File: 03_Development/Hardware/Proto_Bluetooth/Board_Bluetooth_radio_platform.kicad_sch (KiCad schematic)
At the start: 51 parts, among them J1 Conn_01x02, J10 Conn_01x03, J11 HMI_rotaryEncoder_1, J12 HMI_rotaryEncoder_1, J13 Conn_01x08_epaper, J17 Conn_01x02, J19 Conn_01x02_rn52_usb, J2 Conn_01x08, J3 BT_RN52_connector_left, J4 Conn_01x02, J5 BT_RN52_connector_right, J6 FM_interface, J7 BT_debug_connector, J8 BT_extension_connector, J9 SYS_debug_connector, SW1 SW_Push, U1 LM317_TO-220, U2 NXE2S1205MC

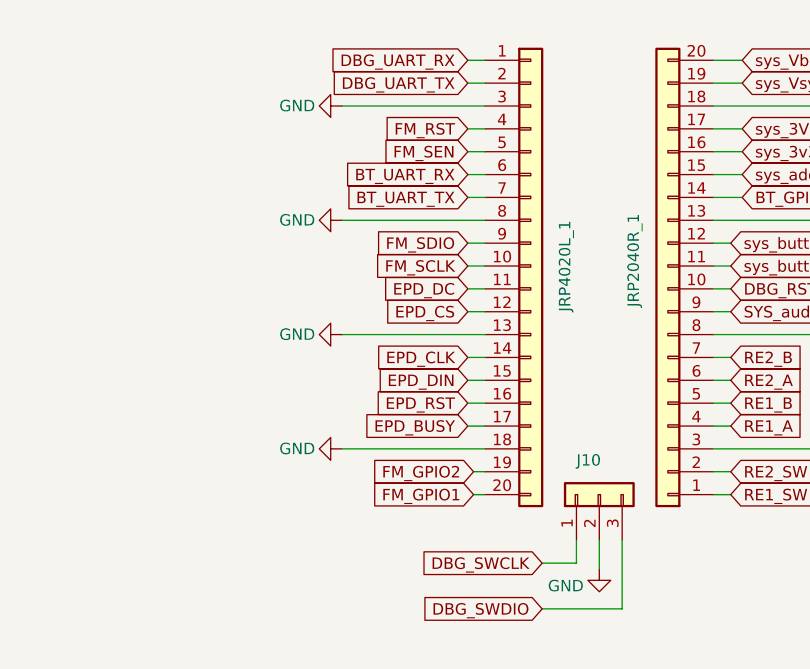
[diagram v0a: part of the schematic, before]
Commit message: [HDW_41] FIX communication lines to central unit
FM, EP and BT modules had been routed to ports of RP2040 which don't allow
UART or I2C and must have been changed
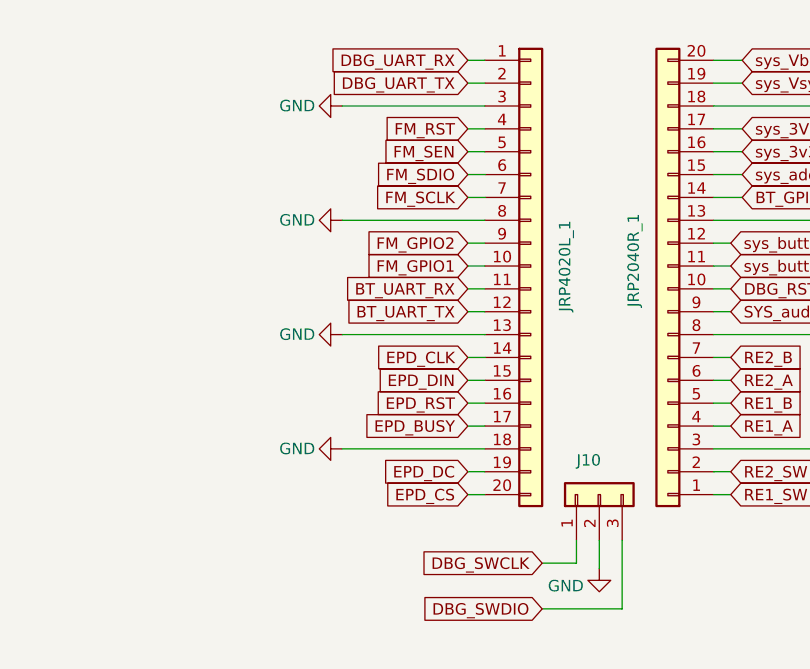
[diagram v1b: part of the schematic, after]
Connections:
- net BT_UART_RX: now also JRP4020L_1.11 (Pin_11); no longer JRP4020L_1.6 (Pin_6)
- net BT_UART_TX: now also JRP4020L_1.12 (Pin_12); no longer JRP4020L_1.7 (Pin_7)
- net EPD_CS: now also JRP4020L_1.20 (Pin_20); no longer JRP4020L_1.12 (Pin_12)
- net EPD_DC: now also JRP4020L_1.19 (Pin_19); no longer JRP4020L_1.11 (Pin_11)
- net FM_GPIO1: now also JRP4020L_1.10 (Pin_10); no longer JRP4020L_1.20 (Pin_20)
- net FM_GPIO2: now also JRP4020L_1.9 (Pin_9); no longer JRP4020L_1.19 (Pin_19)
- net FM_SCLK: now also JRP4020L_1.7 (Pin_7); no longer JRP4020L_1.10 (Pin_10)
- net FM_SDIO: now also JRP4020L_1.6 (Pin_6); no longer JRP4020L_1.9 (Pin_9)
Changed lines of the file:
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@@
     (stroke (width 0) (type default) (color 0 0 0 0))
   )
-  (wire (pts (xy 224.155 146.05) (xy 225.425 146.05))
+  (wire (pts (xy 223.52 146.05) (xy 225.425 146.05))
     (stroke (width 0) (type default) (color 0 0 0 0))
   )
@@
     (stroke (width 0) (type default) (color 0 0 0 0))
   )
-  (wire (pts (xy 224.155 148.59) (xy 225.425 148.59))
+  (wire (pts (xy 223.52 148.59) (xy 225.425 148.59))
     (stroke (width 0) (type default) (color 0 0 0 0))
   )
@@
     (stroke (width 0) (type default) (color 0 0 0 0))
   )
+  (global_label "BT_UART_RX" (shape input) (at 223.52 125.73 180) (fields_autoplaced)
+    (effects (font (size 1.27 1.27)) (justify right))
+    (property "Intersheet References" "${INTERSHEET_REFS}" (id 0) (at 209.7979 125.6506 0)
+      (effects (font (size 1.27 1.27)) (justify right) hide)
+    )
+  )
   (global_label "BT_SPI_SS" (shape input) (at 59.69 178.435 0) (fields_autoplaced)
     (effects (font (size 1.27 1.27)) (justify left))
@@
     )
   )
-  (global_label "BT_UART_RX" (shape input) (at 223.52 113.03 180) (fields_autoplaced)
-    (effects (font (size 1.27 1.27)) (justify right))
-    (property "Intersheet References" "${INTERSHEET_REFS}" (id 0) (at 209.7979 112.9506 0)
-      (effects (font (size 1.27 1.27)) (justify right) hide)
-    )
-  )
   (global_label "FM_SDIO" (shape input) (at 91.44 182.88 180) (fields_autoplaced)
     (effects (font (size 1.27 1.27)) (justify right))
@@
     )
   )
+  (global_label "FM_GPIO1" (shape input) (at 223.52 123.19 180) (fields_autoplaced)
+    (effects (font (size 1.27 1.27)) (justify right))
+    (property "Intersheet References" "${INTERSHEET_REFS}" (id 0) (at 211.9145 123.1106 0)
+      (effects (font (size 1.27 1.27)) (justify right) hide)
+    )
+  )
   (global_label "sys_3V3_EN" (shape input) (at 254 107.95 0) (fields_autoplaced)
     (effects (font (size 1.27 1.27)) (justify left))
@@
     )
   )
-  (global_label "EPD_DC" (shape input) (at 223.52 125.73 180) (fields_autoplaced)
-    (effects (font (size 1.27 1.27)) (justify right))
-    (property "Intersheet References" "${INTERSHEET_REFS}" (id 0) (at 213.9102 125.6506 0)
-      (effects (font (size 1.27 1.27)) (justify right) hide)
-    )
-  )
   (global_label "BT_SPKR_R+" (shape input) (at 59.944 145.415 0) (fields_autoplaced)
     (effects (font (size 1.27 1.27)) (justify left))
@@
     )
   )
-  (global_label "EPD_CS" (shape input) (at 223.52 128.27 180) (fields_autoplaced)
-    (effects (font (size 1.27 1.27)) (justify right))
-    (property "Intersheet References" "${INTERSHEET_REFS}" (id 0) (at 213.9707 128.1906 0)
-      (effects (font (size 1.27 1.27)) (justify right) hide)
-    )
-  )
   (global_label "DBG_RST" (shape input) (at 252.73 125.73 0) (fields_autoplaced)
     (effects (font (size 1.27 1.27)) (justify left))
@@
     )
   )
-  (global_label "FM_GPIO1" (shape input) (at 224.155 148.59 180) (fields_autoplaced)
-    (effects (font (size 1.27 1.27)) (justify right))
-    (property "Intersheet References" "${INTERSHEET_REFS}" (id 0) (at 212.5495 148.5106 0)
-      (effects (font (size 1.27 1.27)) (justify right) hide)
-    )
-  )
   (global_label "FM_GPIO2" (shape input) (at 91.44 170.18 180) (fields_autoplaced)
     (effects (font (size 1.27 1.27)) (justify right))
@@
     )
   )
-  (global_label "FM_SDIO" (shape input) (at 223.52 120.65 180) (fields_autoplaced)
-    (effects (font (size 1.27 1.27)) (justify right))
-    (property "Intersheet References" "${INTERSHEET_REFS}" (id 0) (at 213.1845 120.5706 0)
-      (effects (font (size 1.27 1.27)) (justify right) hide)
-    )
-  )
   (global_label "DBG_SWCLK" (shape input) (at 134.62 186.69 180) (fields_autoplaced)
     (effects (font (size 1.27 1.27)) (justify right))
@@
     )
   )
+  (global_label "FM_GPIO2" (shape input) (at 223.52 120.65 180) (fields_autoplaced)
+    (effects (font (size 1.27 1.27)) (justify right))
+    (property "Intersheet References" "${INTERSHEET_REFS}" (id 0) (at 211.9145 120.5706 0)
+      (effects (font (size 1.27 1.27)) (justify right) hide)
+    )
+  )
   (global_label "BT_MIC_R+" (shape input) (at 59.69 158.115 0) (fields_autoplaced)
     (effects (font (size 1.27 1.27)) (justify left))
@@
     )
   )
+  (global_label "EPD_DC" (shape input) (at 223.52 146.05 180) (fields_autoplaced)
+    (effects (font (size 1.27 1.27)) (justify right))
+    (property "Intersheet References" "${INTERSHEET_REFS}" (id 0) (at 213.9102 145.9706 0)
+      (effects (font (size 1.27 1.27)) (justify right) hide)
+    )
+  )
+  (global_label "FM_SCLK" (shape input) (at 223.52 115.57 180) (fields_autoplaced)
+    (effects (font (size 1.27 1.27)) (justify right))
+    (property "Intersheet References" "${INTERSHEET_REFS}" (id 0) (at 212.8217 115.4906 0)
+      (effects (font (size 1.27 1.27)) (justify right) hide)
+    )
+  )
   (global_label "BT_GPIO6" (shape input) (at 135.89 165.1 180) (fields_autoplaced)
     (effects (font (size 1.27 1.27)) (justify right))
@@
     )
   )
-  (global_label "FM_SCLK" (shape input) (at 223.52 123.19 180) (fields_autoplaced)
-    (effects (font (size 1.27 1.27)) (justify right))
-    (property "Intersheet References" "${INTERSHEET_REFS}" (id 0) (at 212.8217 123.1106 0)
-      (effects (font (size 1.27 1.27)) (justify right) hide)
-    )
-  )
   (global_label "DBG_UART_RX" (shape input) (at 150.495 181.61 0) (fields_autoplaced)
     (effects (font (size 1.27 1.27)) (justify left))
@@
     )
   )
-  (global_label "BT_UART_TX" (shape input) (at 223.52 115.57 180) (fields_autoplaced)
-    (effects (font (size 1.27 1.27)) (justify right))
-    (property "Intersheet References" "${INTERSHEET_REFS}" (id 0) (at 210.1002 115.4906 0)
-      (effects (font (size 1.27 1.27)) (justify right) hide)
-    )
-  )
   (global_label "BT_SPI_SCK" (shape input) (at 59.69 173.355 0) (fields_autoplaced)
     (effects (font (size 1.27 1.27)) (justify left))
@@
     )
   )
+  (global_label "FM_SDIO" (shape input) (at 223.52 113.03 180) (fields_autoplaced)
+    (effects (font (size 1.27 1.27)) (justify right))
+    (property "Intersheet References" "${INTERSHEET_REFS}" (id 0) (at 213.1845 112.9506 0)
+      (effects (font (size 1.27 1.27)) (justify right) hide)
+    )
+  )
   (global_label "BT_GPIO2" (shape input) (at 39.37 145.415 180) (fields_autoplaced)
     (effects (font (size 1.27 1.27)) (justify right))
@@
     )
   )
+  (global_label "EPD_CS" (shape input) (at 223.52 148.59 180) (fields_autoplaced)
+    (effects (font (size 1.27 1.27)) (justify right))
+    (property "Intersheet References" "${INTERSHEET_REFS}" (id 0) (at 213.9707 148.5106 0)
+      (effects (font (size 1.27 1.27)) (justify right) hide)
+    )
+  )
   (global_label "SYS_audio_sw" (shape input) (at 252.73 128.27 0) (fields_autoplaced)
     (effects (font (size 1.27 1.27)) (justify left))
@@
     )
   )
-  (global_label "FM_GPIO2" (shape input) (at 224.155 146.05 180) (fields_autoplaced)
-    (effects (font (size 1.27 1.27)) (justify right))
-    (property "Intersheet References" "${INTERSHEET_REFS}" (id 0) (at 212.5495 145.9706 0)
-      (effects (font (size 1.27 1.27)) (justify right) hide)
-    )
-  )
   (global_label "BT_UART_RTS" (shape input) (at 39.878 173.355 180) (fields_autoplaced)
     (effects (font (size 1.27 1.27)) (justify right))
@@
       (effects (font (size 1.27 1.27)) (justify right) hide)
     )
+  )
+  (global_label "BT_UART_TX" (shape input) (at 223.52 128.27 180) (fields_autoplaced)
+    (effects (font (size 1.27 1.27)) (justify right))
+    (property "Intersheet References" "${INTERSHEET_REFS}" (id 0) (at 210.1002 128.1906 0)
+      (effects (font (size 1.27 1.27)) (justify right) hide)
+    )
